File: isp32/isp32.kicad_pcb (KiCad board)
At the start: 2 copper layers, 55.5 x 48.5 mm, 99 parts, among them J1 BAT1, J10 LoRa_ANT, J12 Micro_SD_Card, J2 Switching, J3 USB_C_Receptacle_USB2.0, J4 ESP_JTAG, J5 GPS_ANT, J6 F0, J7 F1, J9 ANT, M1 Motor_Servo, M2 Motor_Servo, M3 Motor_Servo, M4 Motor_Servo, Q1 BSS138, Q2 BSS138, Q3 IRLML6402, Q4 BSS138, Q5 IRLML6402, Q6 S8050, SW1 RST, SW2 IO0, U1 SC189ZSKTRT, U10 BMP280, U11 MPU-9250, U2 USBLC6-2SC6, U3 STM32F030F4Px, U4 MP1660GTF-Z, U6 24LC32, U7 NEO-XM, U8 ESP32-S3-WROOM-1U, U9 RFM98W-315S2

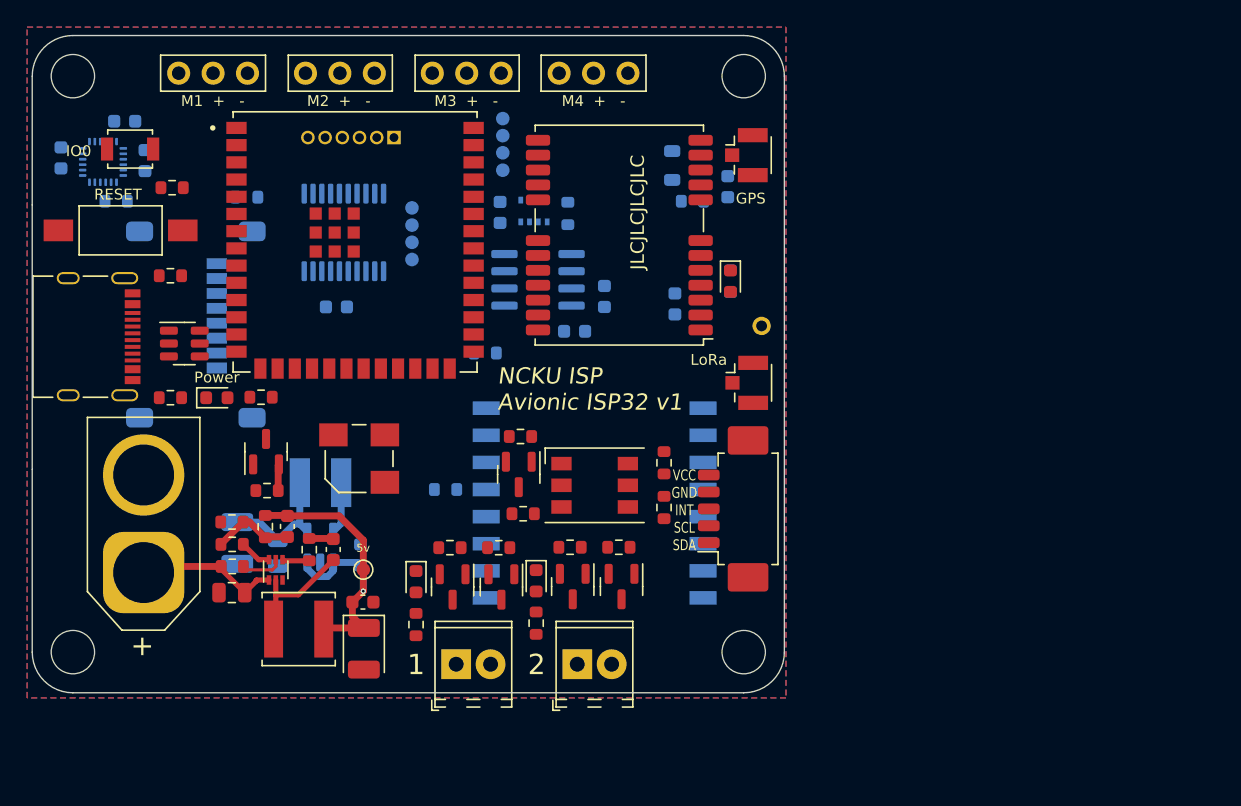
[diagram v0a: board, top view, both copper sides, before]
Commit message: Rough route
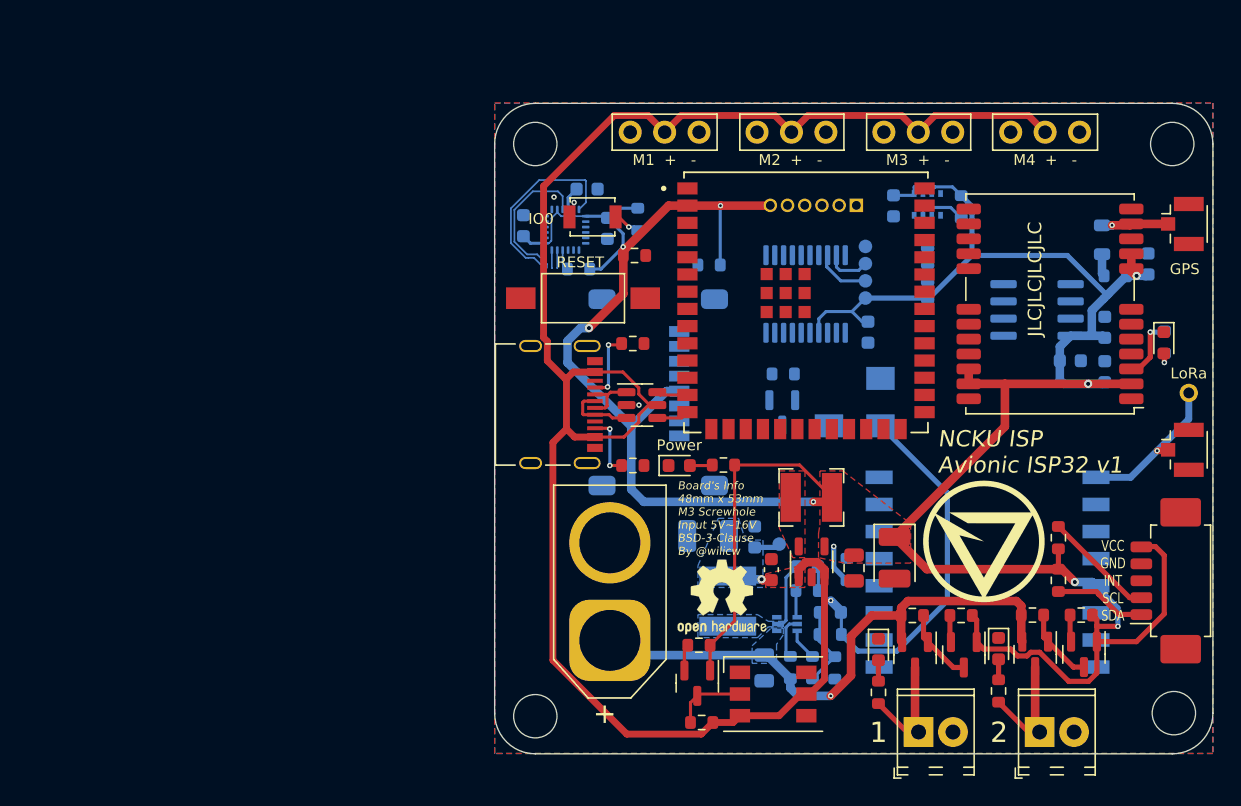
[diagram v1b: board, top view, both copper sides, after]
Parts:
- added REF**: OSHW-Logo2_7.3x6mm_SilkScreen, Symbol:OSHW-Logo2_7.3x6mm_SilkScreen, F.Cu at (110.5, 79.2)
- C1, C10, C6, G***, L1, U1: moved to F.Cu
- C2, C4, C5, C7, C8, L3, LS1, Q6, R10, R11, R3, R33, R8, R9, TP2, U4: moved to B.Cu
- U3: value STM32F030F4Px -> STM32G030F6
- moved C10 48.5 mm to (123.2, 76.3)
- moved R10 45.8 mm to (118.8, 84.4), turned to -90 degrees
- moved G*** 45.7 mm to (129.8, 75.1), turned to 0 degrees
- moved R9 43.8 mm to (117.2, 84.4), turned to -90 degrees
- moved C6 42.5 mm to (120.2, 77.1)
- moved R11 42.4 mm to (118.5, 82.0), turned to 0 degrees
- moved R3 41.9 mm to (115.5, 84.4), turned to 90 degrees
- moved C7 40.6 mm to (118.5, 80.3), turned to 0 degrees
- moved C5 39.7 mm to (113.6, 84.4), turned to -90 degrees
- moved C3 39.3 mm to (121.3, 59.7), turned to -90 degrees
- moved R33 39.1 mm to (115.0, 62.7)
- moved Q6 38.2 mm to (114.9, 65.6), turned to -90 degrees
- moved U4 37.9 mm to (115.3, 81.2), turned to 0 degrees
- moved C13 37.0 mm to (138.7, 59.3)
- moved U6 36.9 mm to (133.7, 58.0)
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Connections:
- U3 pad 1: GND -> SCL
- U3 pad 11: unconnected-(U3-Pad11) -> SERVO0
- U3 pad 12: unconnected-(U3-Pad12) -> SERVO1
- U3 pad 13: unconnected-(U3-Pad13) -> SERVO2
- U3 pad 14: unconnected-(U3-Pad14) -> SERVO3
- U3 pad 15: GND -> unconnected-(U3-Pad15)
- U3 pad 16: +3V3 -> unconnected-(U3-Pad16)
- U3 pad 17: SCL -> unconnected-(U3-Pad17)
- U3 pad 18: SDA -> SWDIO
- U3 pad 19: SWDIO -> SWCLK
- U3 pad 2: unconnected-(U3-Pad2) -> SDA
- U3 pad 20: SWCLK -> unconnected-(U3-Pad20)
- U3 pad 4: RST -> +3V3
- U3 pad 5: +3V3 -> GND
- U3 pad 6: SERVO0 -> RST
- U3 pad 7: SERVO1 -> Buzz
- U3 pad 8: SERVO2 -> RGB
- U3 pad 9: SERVO3 -> unconnected-(U3-Pad9)
- U8 pad 39: Buzz -> unconnected-(U8-Pad39)
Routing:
- net +3V3: track 9.51 -> 239.7 mm, vias 0 -> 9
- net +5V: track 25.5 -> 163.7 mm, vias 1 -> 2
- net +BATT: track 10.8 -> 42.2 mm, vias 0 -> 1
- net IMU_INT: track 0.00 -> 14.4 mm
- net Net-(J10-Pad1): track 0.00 -> 11.4 mm, vias 0 -> 1
- net MISO: track 0.00 -> 11.0 mm
- net Net-(J6-Pad1): track 0.00 -> 8.88 mm
- net Net-(J7-Pad1): track 0.00 -> 8.70 mm
- net SCL: track 0.00 -> 8.30 mm
- net SDA: track 0.00 -> 6.84 mm
- net Net-(Q1-Pad3): track 0.00 -> 5.52 mm
- net Net-(Q4-Pad3): track 0.00 -> 5.52 mm
- net Net-(D3-Pad2): track 0.00 -> 5.38 mm
- net UD+: track 0.00 -> 5.15 mm
- net cc1: track 0.00 -> 5.09 mm, vias 0 -> 2
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- added copper zone on F.Cu, net +3V3
- added copper zone on B.Cu, net +5V
- added copper zone on F.Cu, net +5V
- added copper zone on B.Cu, net +BATT
- added copper zone on B.Cu, net Net-(C4-Pad2)
- added copper zone on F.Cu, net Net-(L1-Pad1)
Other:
- board size 55.5 x 48.5 mm -> 53 x 48 mm
- board text added: "Board's Info 48mm x 53mm M3 Screwhole Input 5V~16V BSD-3-Clause By @wilicw"
